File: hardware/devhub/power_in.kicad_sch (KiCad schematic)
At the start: 28 parts, among them J1 USB-C PWR IN, U1 AP7361C-33E, U13 TPS259470ARPWR

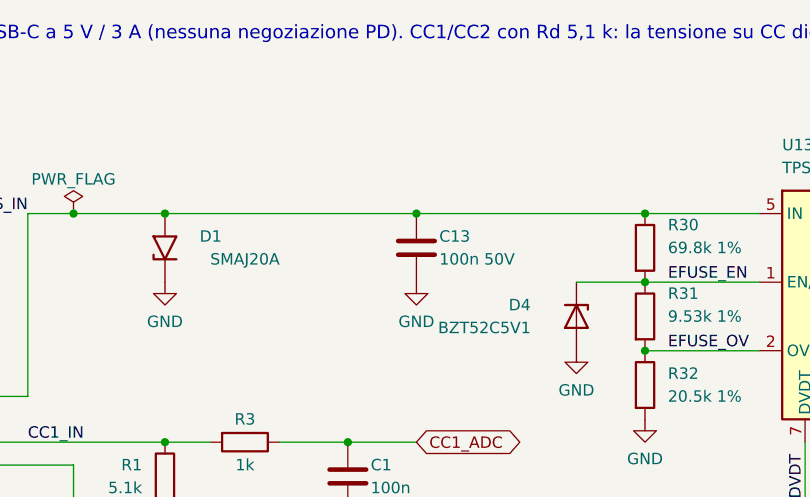
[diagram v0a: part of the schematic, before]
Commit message: Intial PCB layout
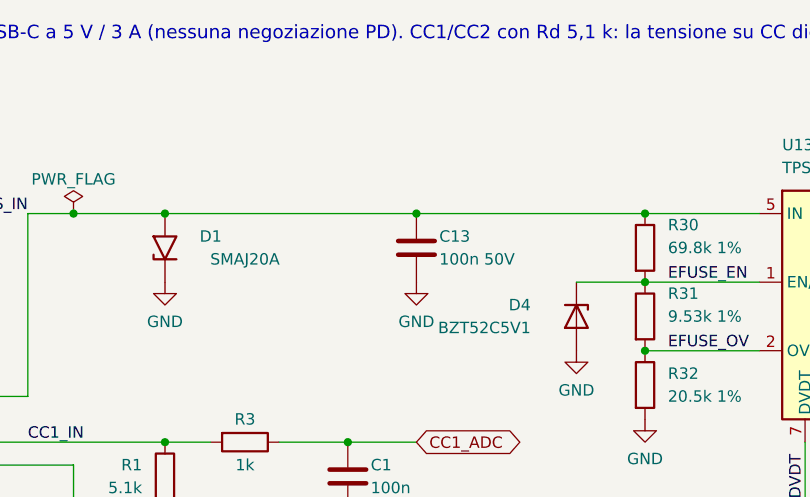
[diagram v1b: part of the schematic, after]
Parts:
- U13: footprint (none) -> lcsc_footprints:C3662799_VQFN-10_L2_0-W2_0-P0_45-TL
